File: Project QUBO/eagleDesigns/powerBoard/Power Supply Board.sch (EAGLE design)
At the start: 84 parts

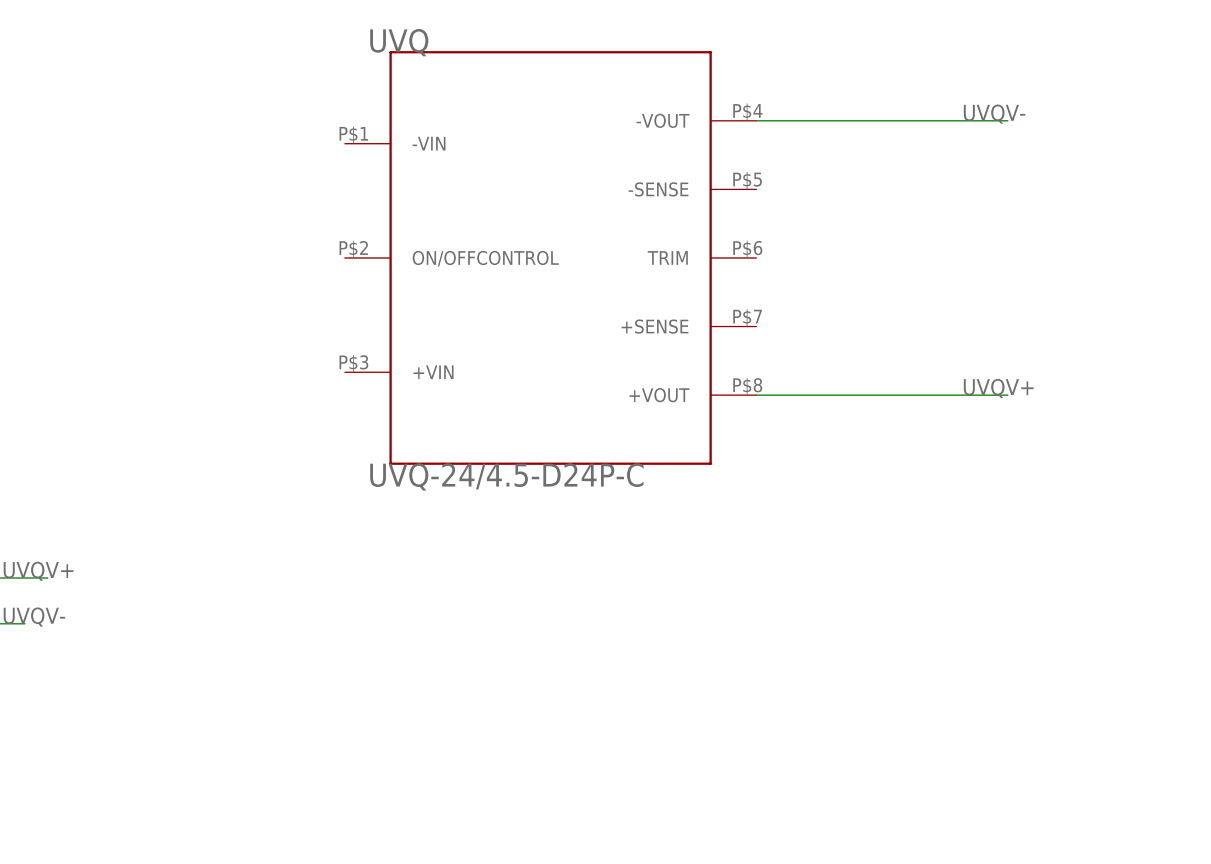
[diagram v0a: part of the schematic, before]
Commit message: edited power supply board sch
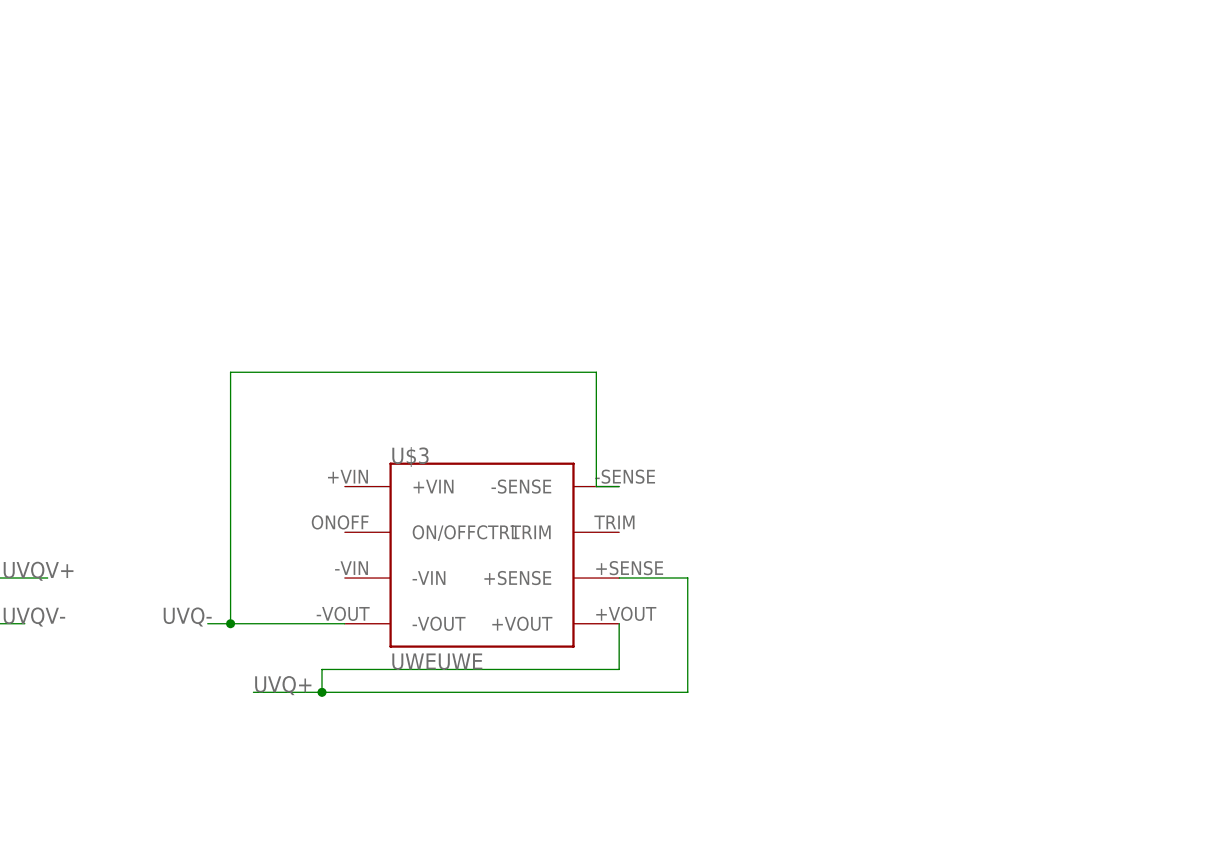
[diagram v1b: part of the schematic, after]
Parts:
- removed UVQ: UVQ-24/4.5-D24P-C, murata:UVQ-24/4.5-D24P-C
- added U$3: UWEUWE, murata:UWEUWE
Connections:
- new net UVQ+: U$3.+SENSE, U$3.+VOUT
- new net UVQ-: U$3.-SENSE, U$3.-VOUT
- net UVQV+: no longer UVQ.+VOUT
- net UVQV-: no longer UVQ.-VOUT
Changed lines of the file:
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@@
 <parts>
 <part name="HOTSWAP1" library="linear" deviceset="LTC4231" device=""/>
-<part name="UVQ" library="murata" deviceset="UVQ-24/4.5-D24P-C" device=""/>
 <part name="DIODE-OR-1" library="linear" deviceset="LTC4359" device=""/>
 <part name="JP1" library="samtec" deviceset="MPSC-01-80" device="MPSC-RA-LC"/>
@@
 <part name="C29" library="resistor" deviceset="C-US" device="C0805" value="10 µF"/>
 <part name="C30" library="resistor" deviceset="CPOL-US" device="D" value="100 uF"/>
+<part name="U$3" library="murata" deviceset="UWE" device="UWE"/>
 </parts>
 <sheets>
@@
 <instances>
 <instance part="HOTSWAP1" gate="G$1" x="134.62" y="48.26"/>
-<instance part="UVQ" gate="G$1" x="12.7" y="144.78"/>
 <instance part="DIODE-OR-1" gate="G$1" x="-25.4" y="45.72"/>
 <instance part="JP1" gate="G$1" x="612.14" y="2.54"/>
@@
 <instance part="C29" gate="G$1" x="327.66" y="-96.52" rot="R90"/>
 <instance part="C30" gate="G$1" x="327.66" y="-104.14" rot="R90"/>
+<instance part="U$3" gate="G$1" x="5.08" y="111.76"/>
 </instances>
 <busses>
@@
 <label x="-48.26" y="109.22" size="1.778" layer="95"/>
 </segment>
-<segment>
-<pinref part="UVQ" gate="G$1" pin="+VOUT"/>
-<wire x1="35.56" y1="129.54" x2="63.5" y2="129.54" width="0.1524" layer="91"/>
-<label x="58.42" y="129.54" size="1.778" layer="95"/>
-</segment>
 </net>
 <net name="UVQV-" class="0">
@@
 <wire x1="-50.8" y1="104.14" x2="-45.72" y2="104.14" width="0.1524" layer="91"/>
 <label x="-48.26" y="104.14" size="1.778" layer="95"/>
-</segment>
-<segment>
-<pinref part="UVQ" gate="G$1" pin="-VOUT"/>
-<wire x1="35.56" y1="160.02" x2="63.5" y2="160.02" width="0.1524" layer="91"/>
-<label x="58.42" y="160.02" size="1.778" layer="95"/>
 </segment>
 </net>
@@
 </segment>
 </net>
+<net name="UVQ-" class="0">
+<segment>
+<pinref part="U$3" gate="G$1" pin="-VOUT"/>
+<wire x1="-10.16" y1="104.14" x2="-22.86" y2="104.14" width="0.1524" layer="91"/>
+<pinref part="U$3" gate="G$1" pin="-SENSE"/>
+<wire x1="20.32" y1="119.38" x2="17.78" y2="119.38" width="0.1524" layer="91"/>
+<wire x1="17.78" y1="119.38" x2="17.78" y2="132.08" width="0.1524" layer="91"/>
+<wire x1="17.78" y1="132.08" x2="-22.86" y2="132.08" width="0.1524" layer="91"/>
+<wire x1="-22.86" y1="132.08" x2="-22.86" y2="104.14" width="0.1524" layer="91"/>
+<wire x1="-22.86" y1="104.14" x2="-25.4" y2="104.14" width="0.1524" layer="91"/>
+<junction x="-22.86" y="104.14"/>
+<label x="-30.48" y="104.14" size="1.778" layer="95"/>
+</segment>
+</net>
+<net name="UVQ+" class="0">
+<segment>
+<pinref part="U$3" gate="G$1" pin="+SENSE"/>
+<wire x1="20.32" y1="109.22" x2="27.94" y2="109.22" width="0.1524" layer="91"/>
+<wire x1="27.94" y1="109.22" x2="27.94" y2="96.52" width="0.1524" layer="91"/>
+<wire x1="27.94" y1="96.52" x2="-12.7" y2="96.52" width="0.1524" layer="91"/>
+<pinref part="U$3" gate="G$1" pin="+VOUT"/>
+<wire x1="-12.7" y1="96.52" x2="-20.32" y2="96.52" width="0.1524" layer="91"/>
+<wire x1="20.32" y1="104.14" x2="20.32" y2="99.06" width="0.1524" layer="91"/>
+<wire x1="20.32" y1="99.06" x2="-12.7" y2="99.06" width="0.1524" layer="91"/>
+<wire x1="-12.7" y1="99.06" x2="-12.7" y2="96.52" width="0.1524" layer="91"/>
+<junction x="-12.7" y="96.52"/>
+<label x="-20.32" y="96.52" size="1.778" layer="95"/>
+</segment>
+</net>
